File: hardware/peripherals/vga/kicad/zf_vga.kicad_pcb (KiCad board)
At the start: 2 copper layers, 143 x 85 mm, 56 parts, among them J2 Z-FIGHTER Expansion Port, SW1 SW_DIP_x03, U1 4040, U10 74HC165, U11 AS6C6264, U12 74HC541, U13 74HC541, U14 74HC541, U2 4040, U3 GAL16V8, U4 GAL16V8, U5 74HC541, U6 74HC541, U7 74HC00, U8 74HC04, U9 74HC74, X1 CXO_DIP14

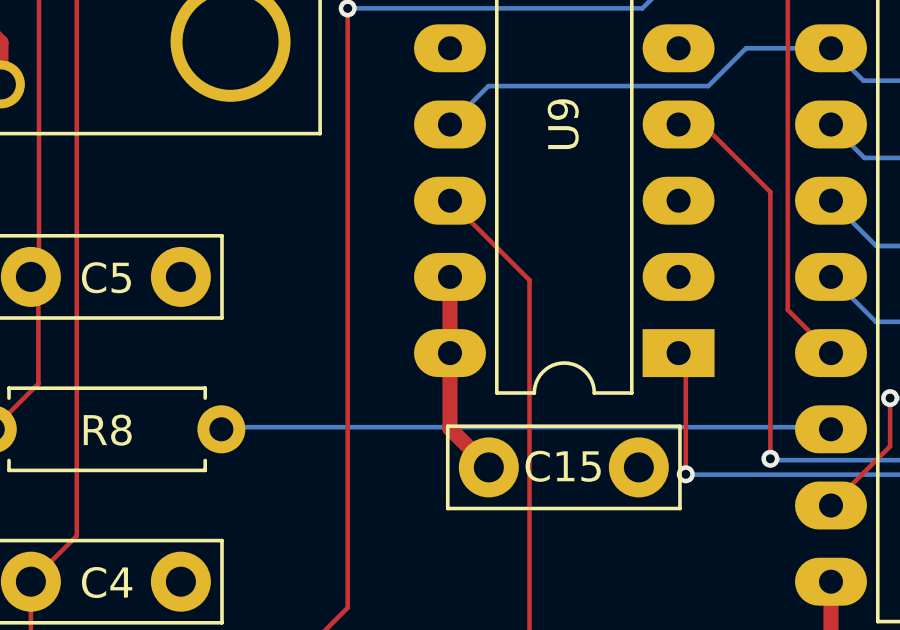
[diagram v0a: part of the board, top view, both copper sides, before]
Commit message: Routing
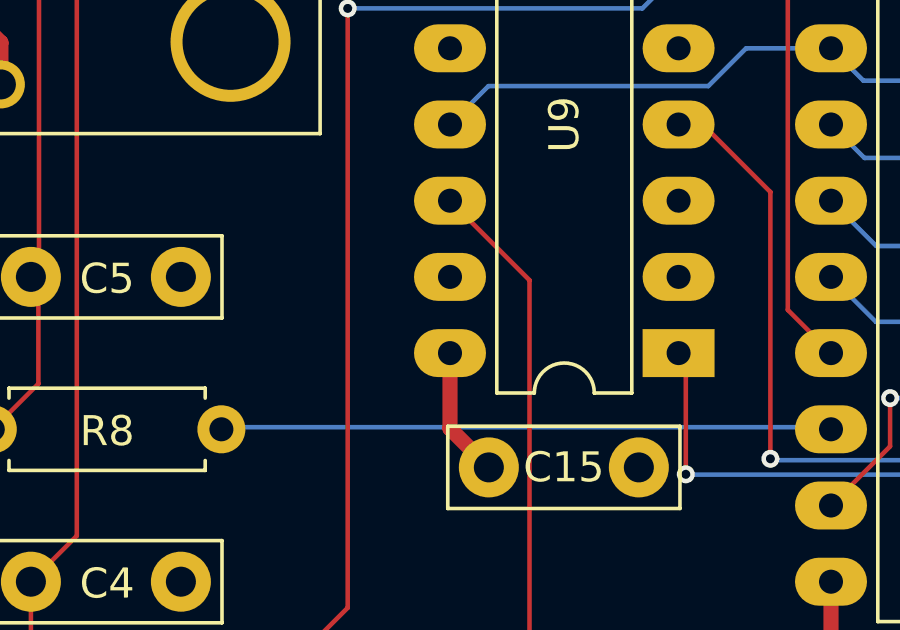
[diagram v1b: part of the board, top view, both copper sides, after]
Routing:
- net VCC: track 82.7 -> 80.1 mm
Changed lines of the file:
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@@
     (thickness 1.6)
     (drawings 15)
-    (tracks 1043)
+    (tracks 1042)
     (zones 0)
     (modules 56)
@@
   (segment (start 146.05 92.699) (end 147.345 93.994) (width 0.508) (layer F.Cu) (net 20))
   (segment (start 90.239 87.644) (end 90.239 90.159) (width 0.508) (layer F.Cu) (net 20))
-  (segment (start 133.419 43.194) (end 133.419 45.734) (width 0.508) (layer F.Cu) (net 20))
   (segment (start 209.619 55.894) (end 210.889 57.164) (width 0.508) (layer F.Cu) (net 20))
   (segment (start 227.119 50.814) (end 222.748999 50.814) (width 1.5) (layer B.Cu) (net 20))
@@
   (segment (start 209.619 73.674) (end 209.489 73.804) (width 0.1524) (layer B.Cu) (net 49))
   (segment (start 209.489 73.804) (end 188.778999 73.804) (width 0.1524) (layer B.Cu) (net 49))
-  (segment (start 146.119 35.574) (end 143.288999 35.574) (width 0.1524) (layer B.Cu) (net 50))
-  (segment (start 142.028999 36.834) (end 134.699 36.834) (width 0.1524) (layer B.Cu) (net 50))
-  (segment (start 143.288999 35.574) (end 142.028999 36.834) (width 0.1524) (layer B.Cu) (net 50))
-  (segment (start 134.699 36.834) (end 133.419 38.114) (width 0.1524) (layer B.Cu) (net 50))
   (segment (start 175.57039 37.08539) (end 179.139 40.654) (width 0.1524) (layer B.Cu) (net 50))
   (segment (start 160.456389 37.08539) (end 175.57039 37.08539) (width 0.1524) (layer B.Cu) (net 50))
@@
   (segment (start 180.17761 41.69261) (end 179.139 40.654) (width 0.1524) (layer B.Cu) (net 50))
   (segment (start 191.839 43.194) (end 190.3376 41.6926) (width 0.1524) (layer B.Cu) (net 50))
+  (segment (start 146.119 35.574) (end 143.288999 35.574) (width 0.1524) (layer B.Cu) (net 50))
+  (segment (start 143.288999 35.574) (end 142.028999 36.834) (width 0.1524) (layer B.Cu) (net 50))
+  (segment (start 142.028999 36.834) (end 134.699 36.834) (width 0.1524) (layer B.Cu) (net 50))
+  (segment (start 134.699 36.834) (end 133.419 38.114) (width 0.1524) (layer B.Cu) (net 50))
   (via (at 186.278999 37.633995) (size 0.6) (drill 0.3) (layers F.Cu B.Cu) (net 51))
   (segment (start 184.219 35.574) (end 186.278995 37.633995) (width 0.1524) (layer F.Cu) (net 51))
